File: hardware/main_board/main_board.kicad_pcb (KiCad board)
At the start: 2 copper layers, 96 x 72 mm, 90 parts, among them IC1 E22-900M22S, IC2 INA226AIDGST, IC3 INA226AIDGST, IC4 TPS2121RUXT, IC5 TP5000-QFN16, J1 power swith, J2 I2C External Modules, J3 Solar panel, J4 WI-FI switch, J5 Battary over BMS, J6 USB4105-GF-A-060, U1 ESP32-C3-WROOM-02, U2 DS3231SN, U4 TPS631000DRLR, U5 PCA9536DR, U6 USBLC6-2SC6

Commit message: hw v1 clean up
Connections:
- net Net-(J4-Pin_1) renamed /main_board/WIFI_SW

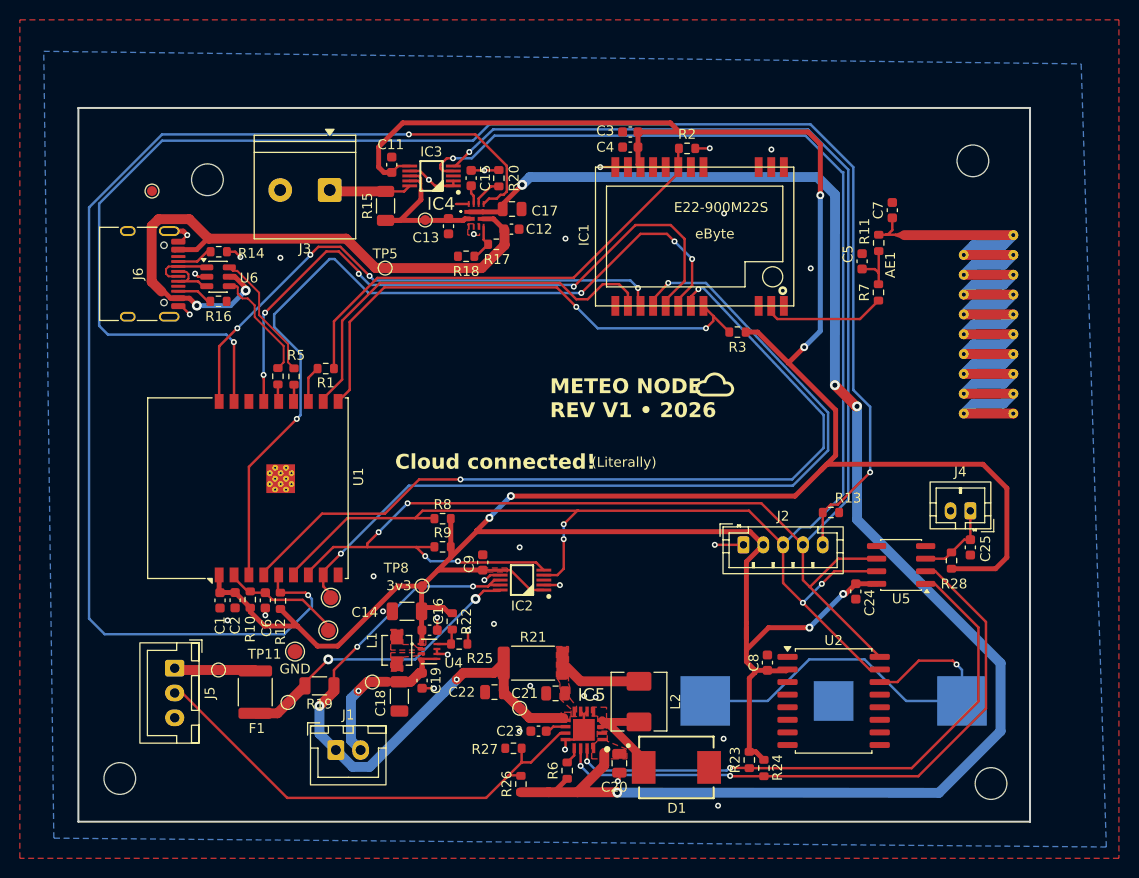
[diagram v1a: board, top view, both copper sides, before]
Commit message: software
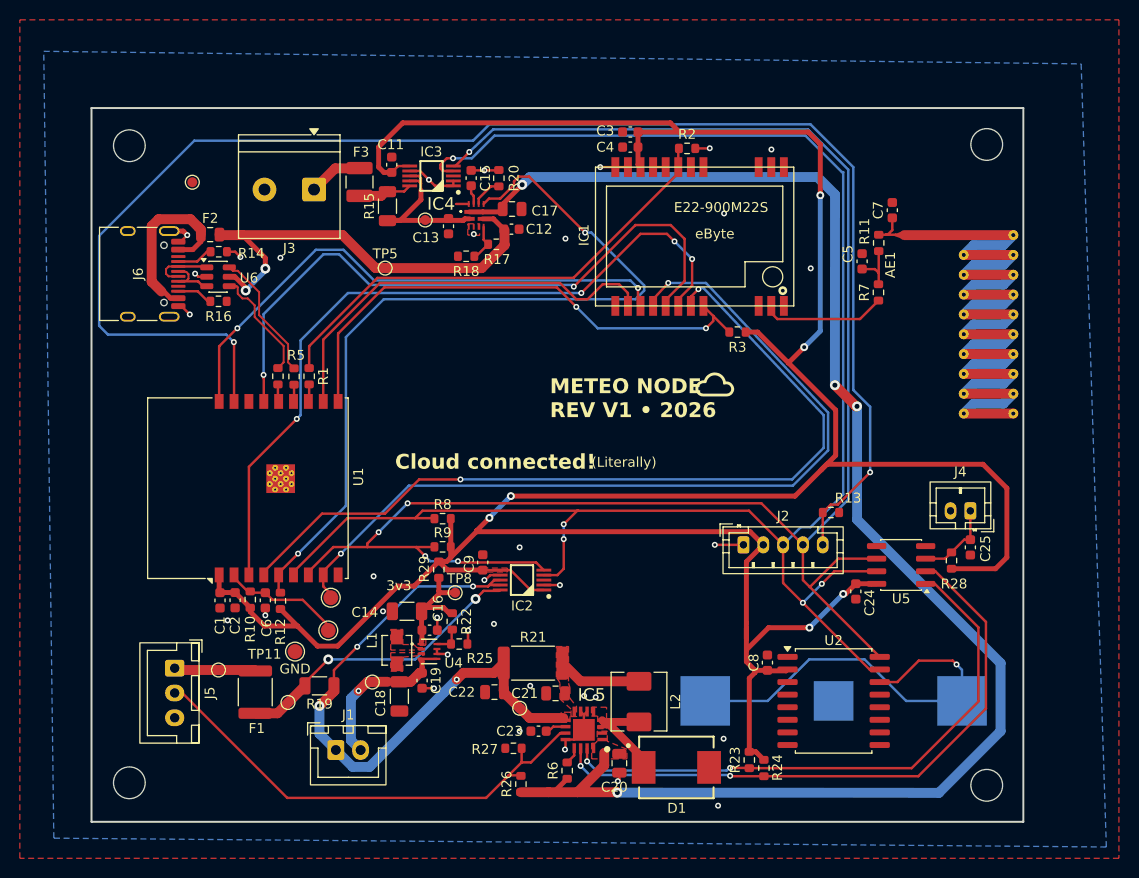
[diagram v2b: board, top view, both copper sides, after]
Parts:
- added F2: 0ZCK0075FF2E, Fuse:Fuse_0805_2012Metric, F.Cu at (115.1, 77.9)
- added F3: 0ZCH0075AF2E, Fuse:Fuse_1210_3225Metric, F.Cu at (130.1, 72.6)
- added R29: 0R, Resistor_SMD:R_0603_1608Metric, F.Cu at (138.2, 111.7)
- R15: value 100mR -> 20mR
- moved REF1 8.59 mm to (106.9, 69.0)
- moved TP9 4.16 mm to (113.3, 72.6)
- moved TP8 3.41 mm to (139.8, 114.0)
- moved REF2 2.16 mm to (193.4, 68.8)
- moved R1 1.85 mm to (125.1, 92.2), turned to -90 degrees
- moved J3 1.59 mm to (125.6, 73.4)
- moved REF4 1.06 mm to (106.9, 133.2)
- moved REF3 0.47 mm to (193.4, 133.5)
- moved R15 0.19 mm to (133.0, 75.1)
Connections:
- C14 pad 1: +3V3 -> Net-(U4-VOUT)
- C16 pad 1: +3V3 -> Net-(U4-VOUT)
- J3 pad 1: SOLAR+ -> Net-(J3-Pin_1)
- J6 pad A4: /Power/USB_5V -> Net-(F2-Pad1)
- J6 pad A9: /Power/USB_5V -> Net-(F2-Pad1)
- J6 pad B4: /Power/USB_5V -> Net-(F2-Pad1)
- J6 pad B9: /Power/USB_5V -> Net-(F2-Pad1)
- R22 pad 1: +3V3 -> Net-(U4-VOUT)
- TP8 pad 1: +3V3 -> Net-(U4-VOUT)
- U4 pad 1: +3V3 -> Net-(U4-VOUT)
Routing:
- net CHARGE_SOURCE_STATUS_OUT: track 123.8 -> 83.3 mm
- net /Power/USB_5V: track 66.2 -> 45.0 mm
- net Net-(F2-Pad1): track 0.00 -> 18.7 mm
- net Net-(U4-VOUT): track 0.00 -> 12.8 mm
- net +3V3: track 309.1 -> 299.7 mm
- net /main_board/SPI_MOSI: track 84.3 -> 76.1 mm
- net Net-(J3-Pin_1): track 0.00 -> 5.48 mm
- net SOLAR+: track 8.69 -> 5.71 mm
- net Net-(U1-IO21/TXD): track 3.70 -> 1.75 mm
- net /main_board/WAKE_IRQ: track 155.0 -> 153.1 mm
- net /main_board/LORA_RXEN: track 48.2 -> 49.2 mm
- net /main_board/SPI_MISO: track 66.2 -> 65.8 mm, vias 4 -> 2
- net /main_board/LORA_BUSY: track 55.6 -> 55.4 mm, vias 4 -> 2
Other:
- board size 96 x 72 mm -> 94 x 72 mm
